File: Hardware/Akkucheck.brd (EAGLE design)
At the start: 21.1 x 17.8 mm, 44 parts, among them IC1 MEGA8-MI, IC2 78L05F

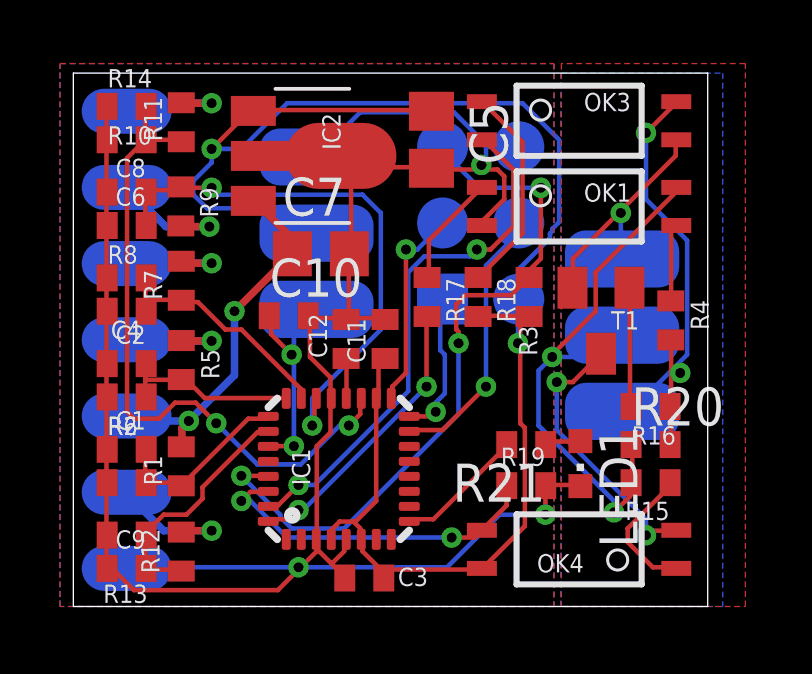
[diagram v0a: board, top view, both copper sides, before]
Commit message: updated BOM
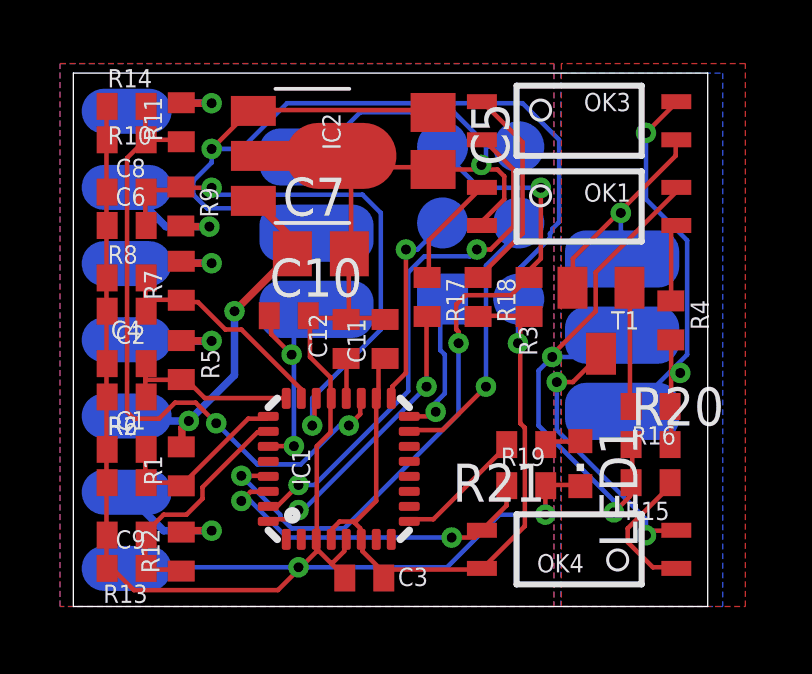
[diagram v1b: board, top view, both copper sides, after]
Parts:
- C5, C7: value (none) -> 2u2
- moved C5 0.07 mm to (11.8, 15.2)
